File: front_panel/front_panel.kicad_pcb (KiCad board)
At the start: 2 copper layers, 68.8 x 19.8 mm, 0 parts

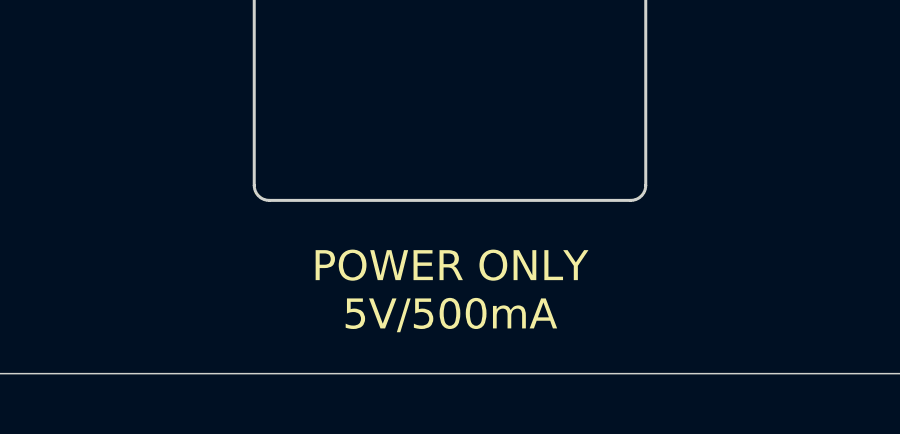
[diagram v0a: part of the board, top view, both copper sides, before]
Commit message: DC current symbol
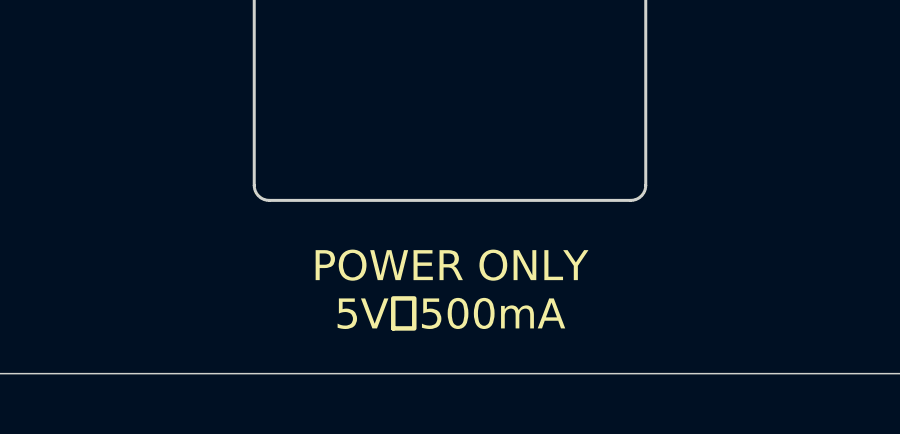
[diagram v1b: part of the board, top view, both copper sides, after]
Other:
- board text added: "POWER ONLY 5V⎓500mA"
- board text removed: "POWER ONLY 5V/500mA"
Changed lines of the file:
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@@
 		(layer "Edge.Cuts")
 	)
-	(gr_text "POWER ONLY\n5V/500mA"
+	(gr_text "POWER ONLY\n5V⎓500mA"
 		(at 110.9 107.15 0)
 		(layer "F.SilkS")
